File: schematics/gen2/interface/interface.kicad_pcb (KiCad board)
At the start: 2 copper layers, 100 x 90.6 mm, 16 parts, among them U1 74LS00, U2 74LS00, U4 74LS245, U5 74LS193, U6 74LS193, U7 74LS193, U8 74LS193

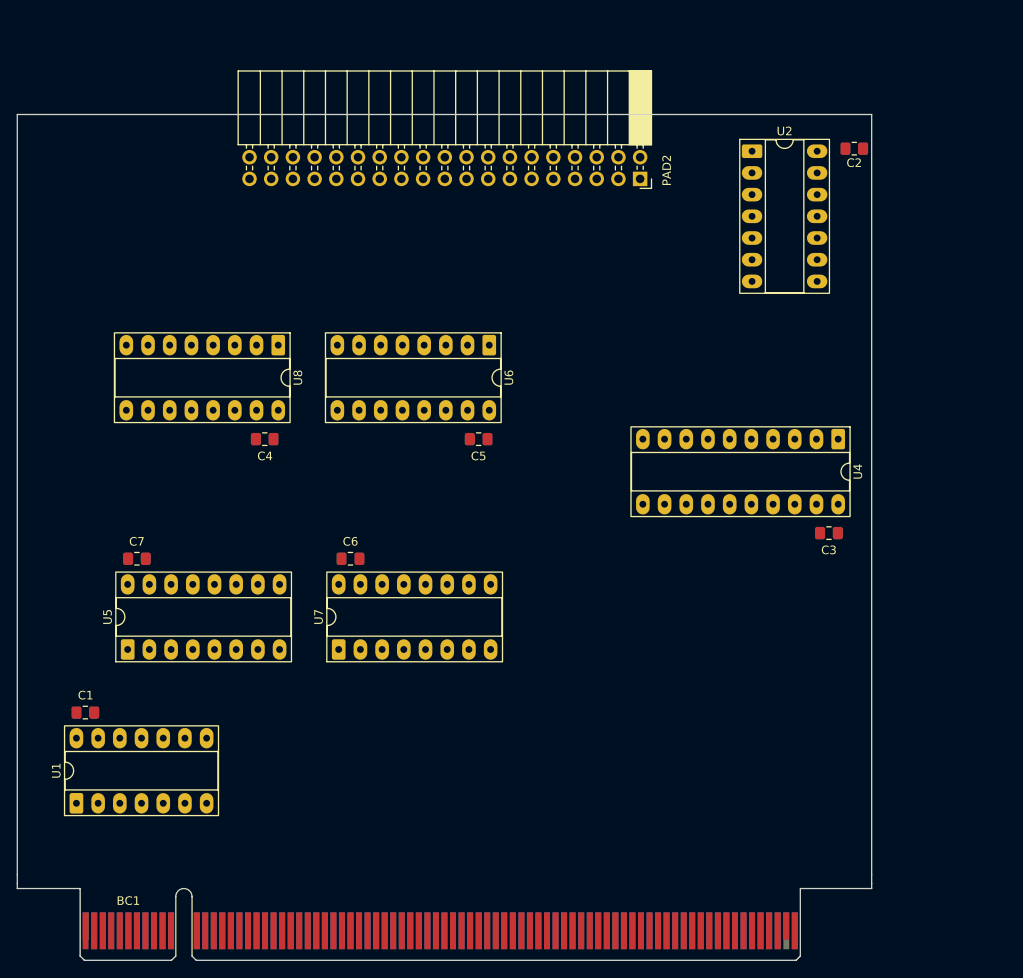
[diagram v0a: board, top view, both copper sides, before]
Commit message: Implement code changes to enhance functionality and improve performance
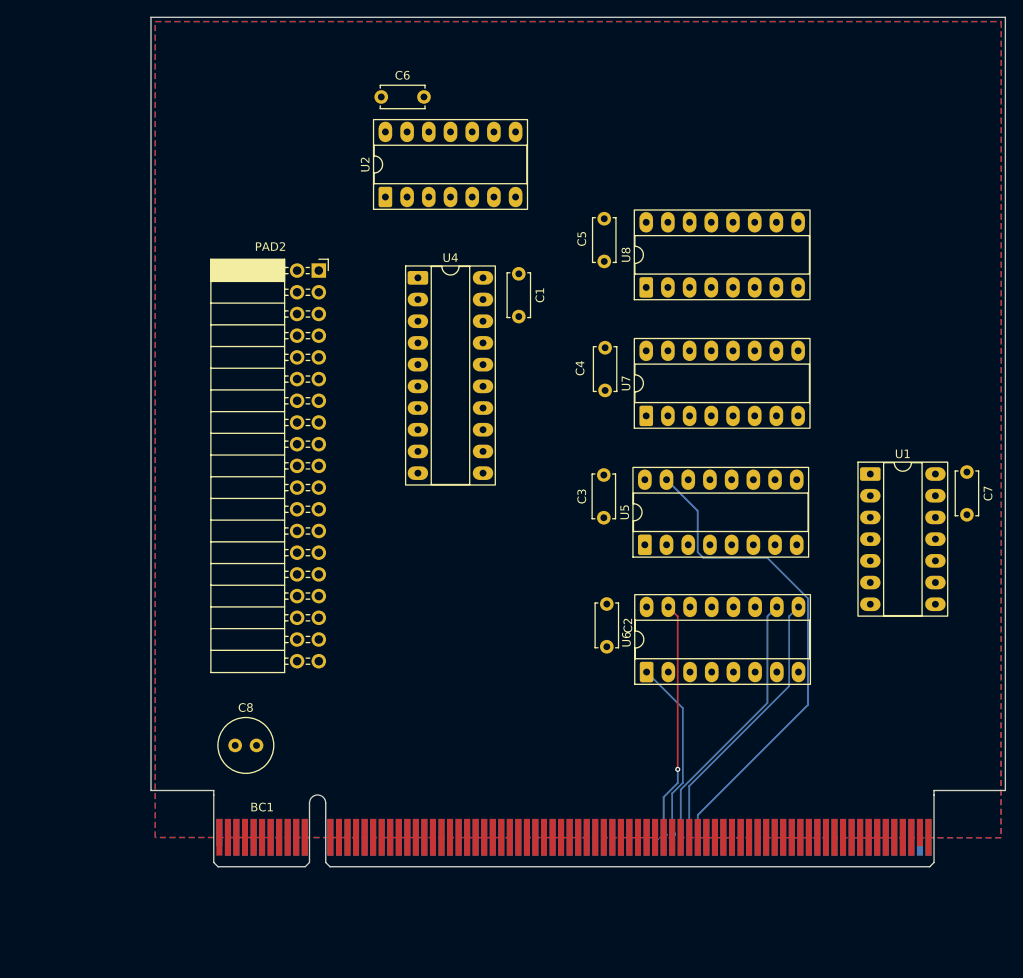
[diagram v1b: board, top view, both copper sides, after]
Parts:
- added C8: C, Capacitor_THT:C_Radial_D6.3mm_H5.0mm_P2.50mm, F.Cu at (95.5, 107.8)
- C1, C2, C3, C4, C5, C6, C7: footprint Capacitor_SMD:C_0805_2012Metric_Pad1.18x1.45mm_HandSolder -> Capacitor_THT:C_Disc_D5.0mm_W2.5mm_P5.00mm
- moved U1 100.6 mm to (169.8, 76.1), turned to 0 degrees
- moved C7 97.7 mm to (181.2, 75.8), turned to -90 degrees
- moved C1 72.2 mm to (128.7, 52.6), turned to -90 degrees
- moved U5 61.8 mm to (143.4, 84.4)
- moved C2 60.7 mm to (139.0, 91.3), turned to -90 degrees
- moved C6 54.2 mm to (112.6, 31.9), turned to 0 degrees
- moved U4 52.7 mm to (116.9, 53.1), turned to 0 degrees
- moved U7 45.2 mm to (143.6, 69.3)
- moved U8 43.6 mm to (143.6, 54.2), turned to 90 degrees
- moved U2 43.2 mm to (113.1, 43.7), turned to 90 degrees
- moved U6 42.5 mm to (143.7, 99.3), turned to 90 degrees
- moved C4 41.2 mm to (138.8, 61.3), turned to -90 degrees
- moved PAD2 39.1 mm to (105.3, 52.3), turned to 0 degrees
- moved C5 29.7 mm to (138.7, 46.2), turned to -90 degrees
- moved C3 27.2 mm to (138.7, 76.2), turned to -90 degrees
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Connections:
- C1 pad 1: GND -> VCC
- C1 pad 2: VCC -> GND
- C2 pad 1: GND -> VCC
- C2 pad 2: VCC -> GND
- C3 pad 1: GND -> VCC
- C3 pad 2: VCC -> GND
- C4 pad 1: GND -> VCC
- C4 pad 2: VCC -> GND
- C5 pad 1: GND -> VCC
- C5 pad 2: VCC -> GND
- C6 pad 1: GND -> VCC
- C6 pad 2: VCC -> GND
- C7 pad 1: GND -> VCC
- C7 pad 2: VCC -> GND
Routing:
- net /BUS4: track 0.00 -> 58.4 mm
- net /BUS3: track 0.00 -> 32.3 mm
- net /BUS2: track 0.00 -> 31.6 mm
- net /BUS0: track 0.00 -> 28.6 mm, vias 0 -> 1
- net /BUS1: track 0.00 -> 22.2 mm
- added copper zone on B.Cu, net GND
- added copper zone on F.Cu, net VCC
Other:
- board size 100 x 90.6 mm -> 100 x 91 mm
